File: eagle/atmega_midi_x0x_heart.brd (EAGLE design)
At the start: 100 x 80 mm, 40 parts, among them J11_VCF_CUTOFF 22-23-2021, U1 ATMEGA328P_PDIP, U2 TLV2372IP

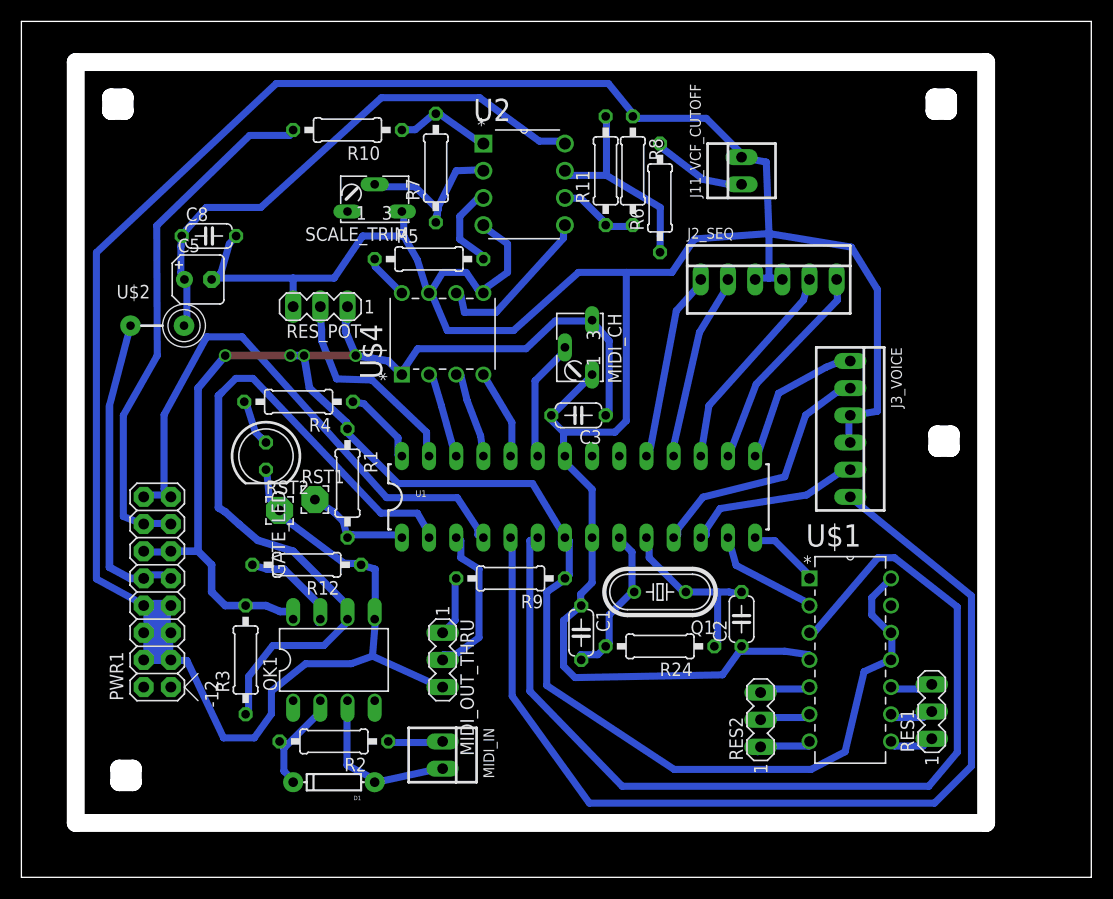
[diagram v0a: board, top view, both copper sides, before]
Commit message: ds1267 is there
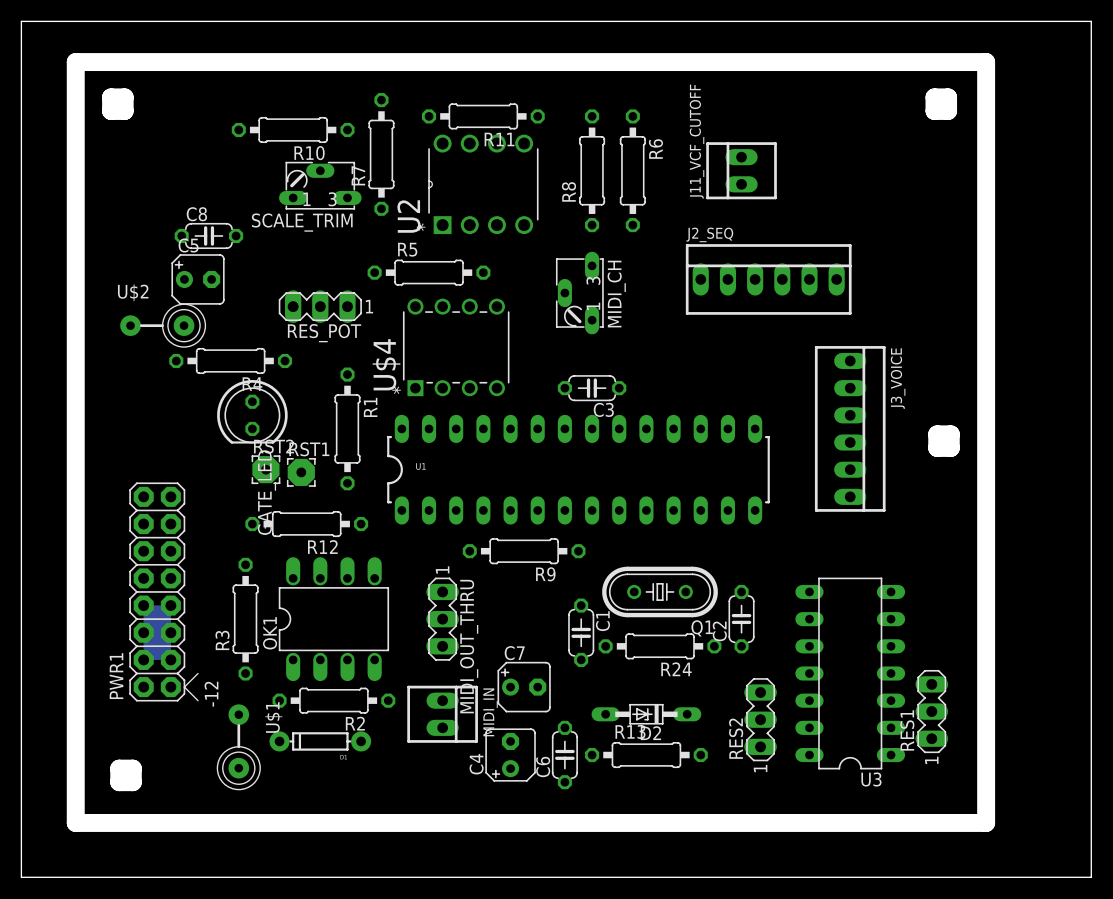
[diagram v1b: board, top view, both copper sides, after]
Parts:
- added C4, C7: 10u, rcl:B45181A
- added C6: 100n, rcl:C050-024X044
- added D2: 5V, diode:DO34Z7
- added R13: 100, rcl:0207/10
- added U3: DS1267S-010+DIP14, Maxim_By_element14_Batch_1:DIP14
- U$1: value MCP42050-E/P -> FB; device MCP42050-E_P:DIP254P762X432-14 -> adafruit:FB
- moved U$1 61.0 mm to (20.3, 12.7), turned to 270 degrees
- moved R11 12.5 mm to (43.2, 71.1), turned to 180 degrees
- moved U2 8.52 mm to (47.0, 68.6), turned to 90 degrees
- moved R4 7.41 mm to (19.6, 48.3)
- moved SCALE_TRIM 5.24 mm to (27.9, 63.5)
- moved R7 5.24 mm to (33.7, 67.6)
- moved R10 5.08 mm to (25.4, 69.8)
- moved MIDI_CH 5.08 mm to (53.3, 54.6)
- moved R1 5.08 mm to (30.5, 41.9)
- moved GATE_LED 4.02 mm to (21.6, 43.2)
- moved RST2 4.02 mm to (22.9, 38.1)
- moved D1 4.02 mm to (27.9, 12.7)
- moved R12 3.81 mm to (26.7, 33.0)
- moved R2 3.81 mm to (29.2, 16.5)
- moved MIDI_IN 3.81 mm to (39.4, 15.2)
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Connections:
- new net -12V: C4.-, C6.2, R13.1, U$1.P$2
- new net N$47: PWR1.1, PWR1.2, U$1.P$1
- new net N$49: C7.-, D2.A, R13.2, U3.1
- net +5V: now also U3.14; no longer U$1.11, U$1.12, U$1.14
- net GND: now also C4.+, C6.1, C7.+, D2.C, U3.7; no longer U$1.4
- net N$22: now also U3.5; no longer U$1.3
- net N$31: now also U3.4; no longer U$1.9
- net N$32: now also U3.2; no longer U$1.8
- net N$33: now also U3.3; no longer U$1.10
- net N$34: now also U3.12; no longer U$1.6
- net N$35: now also U3.11; no longer U$1.7
- net N$36: now also U3.10; no longer U$1.5
- net N$37: now also U3.6; no longer U$1.1
- net N$41: now also U3.8; no longer U$1.2
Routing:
- net GND: track 389.9 -> 0.00 mm
- net +5V: track 190.4 -> 0.00 mm, vias 4 -> 0
- net N$1: track 94.9 -> 0.00 mm
- net N$22: track 92.2 -> 0.00 mm
- net N$30: track 70.0 -> 0.00 mm
- net N$40: track 53.5 -> 0.00 mm
- net +12V: track 51.9 -> 0.00 mm
- net N$15: track 49.1 -> 0.00 mm
- net N$11: track 29.8 -> 0.00 mm
- net N$10: track 24.5 -> 0.00 mm
- net N$23: track 20.1 -> 0.00 mm
- net N$21: track 20.0 -> 0.00 mm
- net N$38: track 19.9 -> 0.00 mm
- net N$17: track 19.6 -> 0.00 mm
- net N$18: track 17.8 -> 0.00 mm
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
